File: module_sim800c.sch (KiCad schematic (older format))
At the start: 31 parts

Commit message: complete schematic
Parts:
- removed J?: LEMO2, symbol LEMO2
- removed P?: simcard, FCI_7111S2015X02LF, symbol 7111S2015X02LF
- J5: renamed from J?; value LEMO2 -> ANTEN
- gave numbers to parts that had none: 28
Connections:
- net labels added: +5V, RXD-01, TXD-01
- net labels removed: 5V, RXD, TXD
- no-connect marks 38 -> 36

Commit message: edit module sim800c
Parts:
- removed C10, C9: 22pF, symbol C
- removed C11, C12: 104, symbol C
- removed C7: C, symbol C
- removed D3: LED, symbol LED
- removed J6: CONN_01X04, symbol CONN_01X04
- removed P2: simcard, FCI_7111S2015X02LF, symbol 7111S2015X02LF
- removed R15: 1K, symbol R
- removed R16: R, symbol R
- removed R18, R19, R20, R21: 5,6K, symbol R
- removed R22, R23: 10K, symbol R
- removed R24: 330, symbol R
- added D3: D_TVS, Diodes_SMD:D_0603, symbol D_TVS
- added J?: SIM_Card, footprint:cardsim, symbol SIM_Card
- added SW1: SW_Push, symbol SW_Push
- added U8: SP1001, footprint:SP1001, symbol SP1001
- C5, C6, C8: footprint (none) -> footprint:C_0603
- D4: footprint (none) -> LEDs:LED_0603
- J7: footprint (none) -> Pin_Headers:Pin_Header_Angled_1x04_Pitch1.27mm
- R12, R13: value 1k -> 100; footprint (none) -> footprint:R_0603
- R14: value 1K -> 100; footprint (none) -> footprint:R_0603
- R17, R25: footprint (none) -> footprint:R_0603
- U3: footprint . -> footprint:sim800c
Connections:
- net labels added: +3V3, CTS, DCD, DTR, RI, RTS
- net labels removed: +5V
- wire segments 47 -> 56
- no-connect marks 36 -> 23
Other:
- moved on the sheet: C6, C8, D4, J7, R17, R25

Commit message: edit module sim800c
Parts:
- removed J?: SIM_Card, footprint:cardsim, symbol SIM_Card
- removed U3: SIM800C-RESCUE-esp32-gateway-hw, footprint:sim800c, symbol SIM800C-RESCUE-esp32-gateway-hw
- removed U8: SP1001, footprint:SP1001, symbol SP1001
- added J?: SIM_Card, symbol SIM_Card
- added U?: SIM800C-RESCUE-esp32-gateway-hw, ., symbol SIM800C-RESCUE-esp32-gateway-hw
- added U?: SP1001, symbol SP1001
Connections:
- wire segments 56 -> 55
- no-connect marks 23 -> 24
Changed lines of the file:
@@
 LIBS:zetex
 LIBS:Zilog
-LIBS:cardslot
 LIBS:esp32-wrover-v3
 LIBS:lm2596
@@
 LIBS:MOSFET-P
 LIBS:OPL-Inductor
-LIBS:sim800c
 LIBS:tc1264
 LIBS:neo-6m
 LIBS:Sim800c
 LIBS:sp1001
-LIBS:sim_card_holder
 LIBS:esp32-gateway-hw-cache
 EELAYER 25 0
@@
 	0    -1   -1   0
 $EndComp
-$Comp
-L SIM800C-RESCUE-esp32-gateway-hw U3
-U 1 1 59DD0550
-P 5850 3300
-F 0 "U3" H 5149 4521 50  0000 L BNN
-F 1 "SIM800C-RESCUE-esp32-gateway-hw" H 5149 1877 50  0000 L BNN
-F 2 "footprint:sim800c" H 7650 2800 50  0001 L BNN
-F 3 "." H 6900 3450 50  0001 L BNN
-F 4 "." H 5550 3800 50  0001 L BNN "Availability"
-F 5 "SIM800C" H 5700 3450 50  0001 L BNN "MP"
-F 6 "." H 5700 3100 50  0001 L BNN "Price"
-F 7 "." H 5750 3100 50  0001 L BNN "Package"
-F 8 "." H 5850 3300 50  0001 L BNN "MF"
-	1    5850 3300
-	1    0    0    -1
-$EndComp
 NoConn ~ 6750 3400
 $Comp
@@
 RI
 $Comp
-L SP1001 U8
-U 1 1 59DD10E8
-P 7500 3550
-F 0 "U8" H 7450 3250 60  0000 C CNN
-F 1 "SP1001" H 7450 4000 60  0000 C CNN
-F 2 "footprint:SP1001" H 7500 3550 60  0001 C CNN
-F 3 "" H 7500 3550 60  0001 C CNN
-	1    7500 3550
-	1    0    0    -1
-$EndComp
-$Comp
 L GND #PWR026
 U 1 1 59DD114F
@@
 	4700 2300 4950 2300
 $Comp
+L SIM800C-RESCUE-esp32-gateway-hw U?
+U 1 1 59DD1931
+P 5850 3300
+F 0 "U?" H 5149 4521 50  0000 L BNN
+F 1 "SIM800C-RESCUE-esp32-gateway-hw" H 5149 1877 50  0000 L BNN
+F 2 "." H 7650 2800 50  0001 L BNN
+F 3 "." H 6900 3450 50  0001 L BNN
+F 4 "." H 5550 3800 50  0001 L BNN "Availability"
+F 5 "SIM800C" H 5700 3450 50  0001 L BNN "MP"
+F 6 "." H 5700 3100 50  0001 L BNN "Price"
+F 7 "." H 5750 3100 50  0001 L BNN "Package"
+F 8 "." H 5850 3300 50  0001 L BNN "MF"
+	1    5850 3300
+	1    0    0    -1
+$EndComp
+$Comp
 L SIM_Card J?
-U 1 1 59DD0C98
+U 1 1 59DD1A9A
 P 8350 2900
-AR Path="/59DD0C98" Ref="J?"  Part="1"
-AR Path="/59DC8035/59DD0C98" Ref="J?"  Part="1"
 F 0 "J?" H 8250 3400 50  0000 R CNN
 F 1 "SIM_Card" H 8300 3300 50  0000 R CNN
-F 2 "footprint:cardsim" H 8350 3250 50  0000 C CNN
+F 2 "" H 8350 3250 50  0000 C CNN
 F 3 "" H 8300 2900 50  0000 C CNN
 	1    8350 2900
 	1    0    0    -1
 $EndComp
-Wire Wire Line
-	7850 3100 7850 3000
+NoConn ~ 7850 3000
+$Comp
+L SP1001 U?
+U 1 1 59DD1ECF
+P 7500 3550
+F 0 "U?" H 7450 3250 60  0000 C CNN
+F 1 "SP1001" H 7450 4000 60  0000 C CNN
+F 2 "" H 7500 3550 60  0001 C CNN
+F 3 "" H 7500 3550 60  0001 C CNN
+	1    7500 3550
+	1    0    0    -1
+$EndComp
 $EndSCHEMATC

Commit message: fix mach nap
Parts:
- J5: symbol LEMO2 -> LEMO2-RESCUE-esp32-gateway-hw
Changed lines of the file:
@@
 LIBS:contrib
 LIBS:valves
+LIBS:esp32-wrover-v3
 LIBS:Symbols_DCDC-ACDC-Converter_RevC_20Jul2012
 LIBS:Symbols_EN60617_13Mar2013
@@
 LIBS:ftdi
 LIBS:gennum
+LIBS:graphic_symbols
 LIBS:hc11
+LIBS:infineon
+LIBS:intersil
 LIBS:ir
 LIBS:Lattice
 LIBS:leds
+LIBS:LEM
+LIBS:logic_programmable
 LIBS:maxim
 LIBS:mechanical
@@
 LIBS:relays
 LIBS:rfcom
+LIBS:RFSolutions
 LIBS:sensors
 LIBS:silabs
@@
 LIBS:zetex
 LIBS:Zilog
-LIBS:esp32-wrover-v3
+LIBS:CP2102
+LIBS:ESP8266
+LIBS:esp-uno
+LIBS:esp-wroom-32
+LIBS:microsd_socket
+LIBS:microsd_spi_cd
+LIBS:MOSFET-N
+LIBS:MOSFET-P
+LIBS:open-project
+LIBS:tc1264
+LIBS:tom_kicad
+LIBS:usb-b
+LIBS:usb_mini_b
+LIBS:w_device
 LIBS:lm2596
 LIBS:mcp73831
-LIBS:MOSFET-P
 LIBS:OPL-Inductor
-LIBS:tc1264
 LIBS:neo-6m
 LIBS:Sim800c
@@
 $EndComp
 $Comp
-L LEMO2 J5
+L LEMO2-RESCUE-esp32-gateway-hw J5
 U 1 1 59DC618A
 P 3700 4000
+AR Path="/59DC618A" Ref="J5"  Part="1"
+AR Path="/59DC8035/59DC618A" Ref="J5"  Part="1"
 F 0 "J5" H 3700 4200 50  0000 C CNN
 F 1 "ANTEN" H 3700 3800 50  0000 C CNN

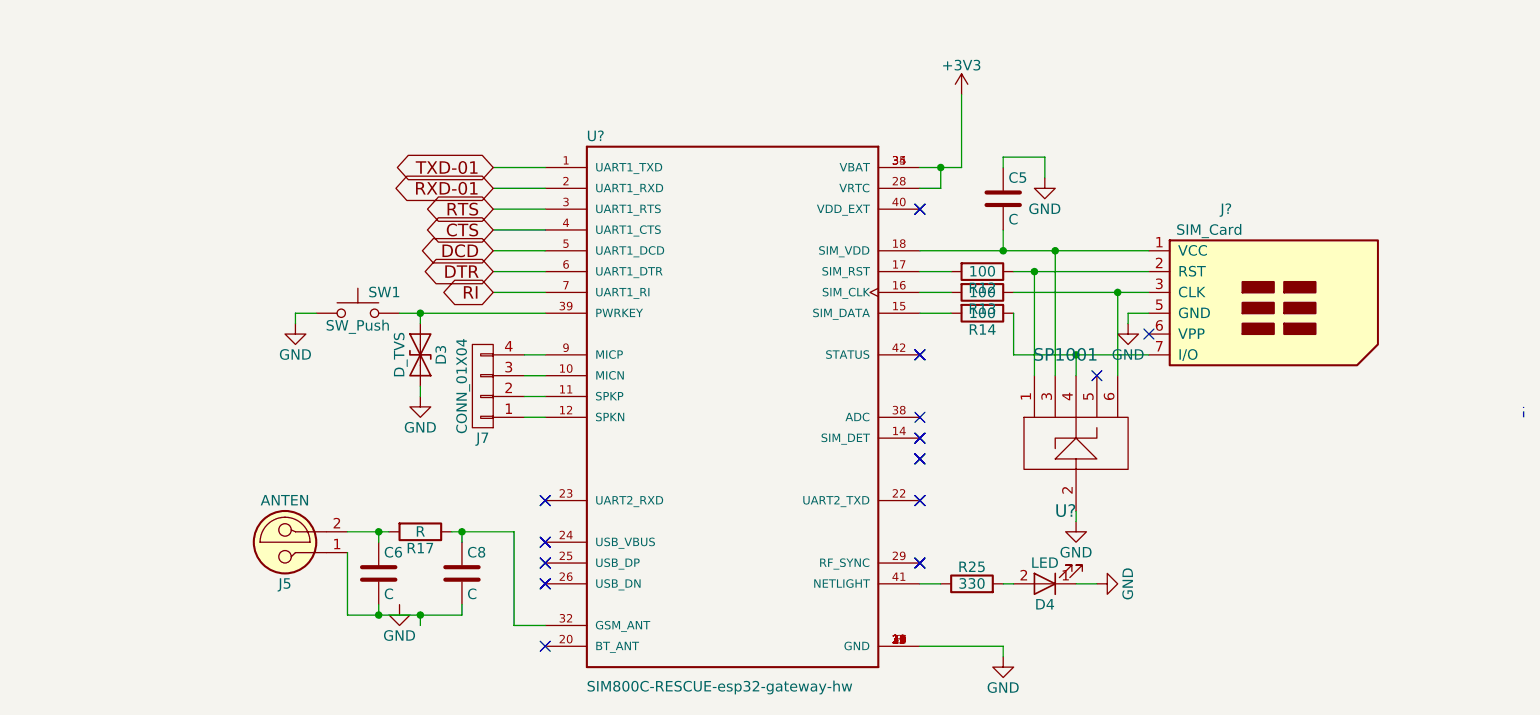
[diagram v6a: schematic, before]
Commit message: update layout
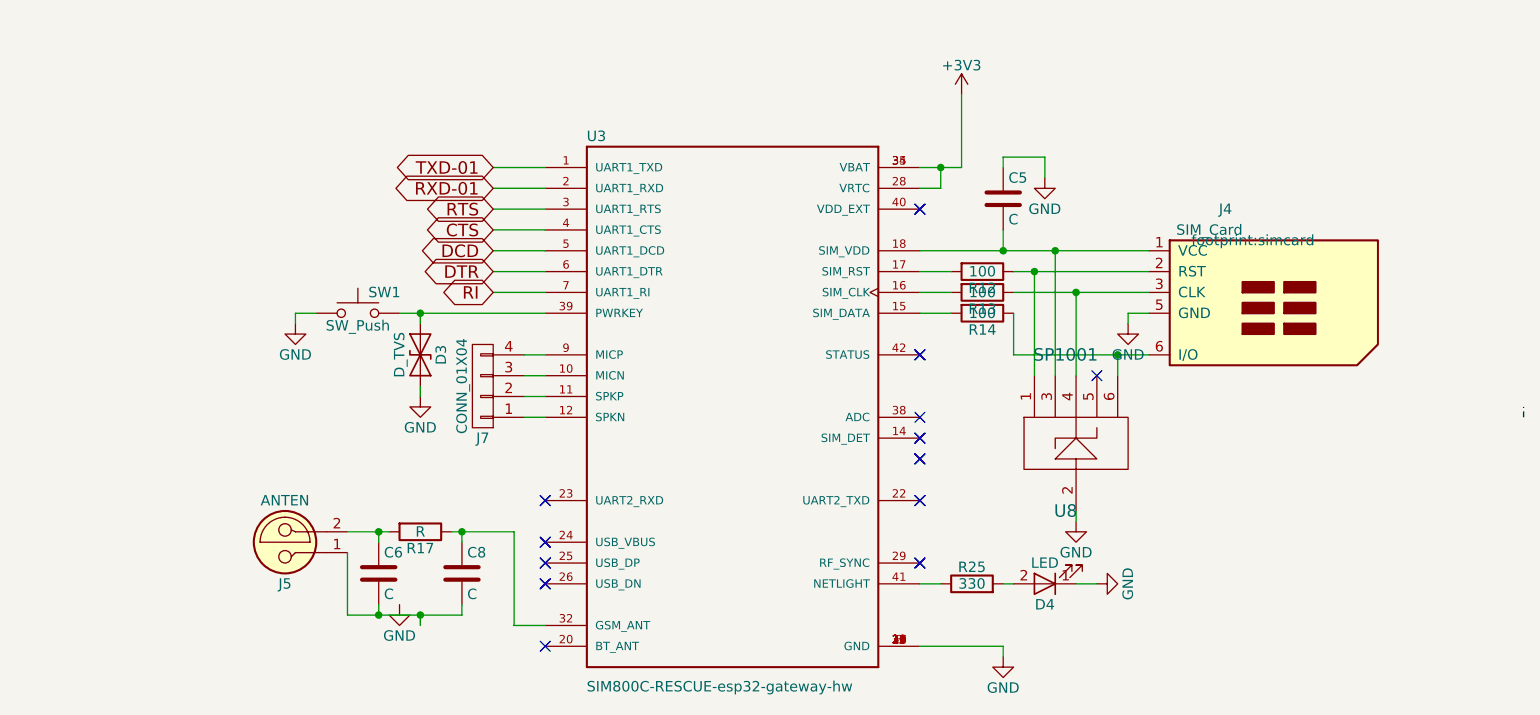
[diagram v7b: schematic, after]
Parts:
- removed J?: SIM_Card, symbol SIM_Card
- added J4: SIM_Card, footprint:simcard, symbol SIM_Card-RESCUE-esp32-gateway-hw
- D3: footprint Diodes_SMD:D_0603 -> Diodes_SMD:D_1206
- J5: footprint (none) -> Pin_Headers:Pin_Header_Straight_1x02_Pitch1.00mm
- SW1: footprint (none) -> footprint:Tact_Switch_TS6X3.6
- U3: renamed from U?; footprint . -> footprint:sim800c
- U8: renamed from U?; footprint (none) -> footprint:SP1001
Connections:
- net GND: now also J4.5 (GND)
- net at R12.1, U8.1: now also J4.2 (RST)
- net at R13.1: now also U8.4, J4.3 (CLK); no longer U8.6
- net at R14.1: now also U8.6, J4.6 (I/O); no longer U8.4
- net at C5.2, U3.18 (SIM_VDD), U8.3: now also J4.1 (VCC)
- no-connect marks 24 -> 23
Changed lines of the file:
@@
 LIBS:contrib
 LIBS:valves
-LIBS:esp32-wrover-v3
 LIBS:Symbols_DCDC-ACDC-Converter_RevC_20Jul2012
 LIBS:Symbols_EN60617_13Mar2013
@@
 LIBS:ftdi
 LIBS:gennum
-LIBS:graphic_symbols
 LIBS:hc11
-LIBS:infineon
-LIBS:intersil
 LIBS:ir
 LIBS:Lattice
 LIBS:leds
-LIBS:LEM
-LIBS:logic_programmable
 LIBS:maxim
 LIBS:mechanical
@@
 LIBS:relays
 LIBS:rfcom
-LIBS:RFSolutions
 LIBS:sensors
 LIBS:silabs
@@
 LIBS:zetex
 LIBS:Zilog
-LIBS:CP2102
-LIBS:ESP8266
-LIBS:esp-uno
-LIBS:esp-wroom-32
-LIBS:microsd_socket
-LIBS:microsd_spi_cd
-LIBS:MOSFET-N
-LIBS:MOSFET-P
-LIBS:open-project
-LIBS:tc1264
-LIBS:tom_kicad
-LIBS:usb-b
-LIBS:usb_mini_b
-LIBS:w_device
+LIBS:esp32-wrover-v3
 LIBS:lm2596
 LIBS:mcp73831
+LIBS:MOSFET-P
 LIBS:OPL-Inductor
+LIBS:tc1264
 LIBS:neo-6m
 LIBS:Sim800c
+LIBS:sim_card_holder
 LIBS:sp1001
 LIBS:esp32-gateway-hw-cache
@@
 $Descr A4 11693 8268
 encoding utf-8
-Sheet 3 4
+Sheet 2 4
 Title ""
 Date ""
@@
 NoConn ~ 6750 3800
 $Comp
-L GND #PWR020
+L GND #PWR010
 U 1 1 59DC6183
 P 7150 4550
-F 0 "#PWR020" H 7150 4300 50  0001 C CNN
+F 0 "#PWR010" H 7150 4300 50  0001 C CNN
 F 1 "GND" H 7150 4400 50  0000 C CNN
 F 2 "" H 7150 4550 50  0001 C CNN
@@
 $EndComp
 $Comp
-L GND #PWR021
+L GND #PWR011
 U 1 1 59DC6189
 P 4250 4300
-F 0 "#PWR021" H 4250 4050 50  0001 C CNN
+F 0 "#PWR011" H 4250 4050 50  0001 C CNN
 F 1 "GND" H 4250 4150 50  0000 C CNN
 F 2 "" H 4250 4300 50  0001 C CNN
@@
 AR Path="/59DC618A" Ref="J5"  Part="1"
 AR Path="/59DC8035/59DC618A" Ref="J5"  Part="1"
+AR Path="/59DDD837/59DC618A" Ref="J5"  Part="1"
+AR Path="/59DDC248/59DC618A" Ref="J5"  Part="1"
 F 0 "J5" H 3700 4200 50  0000 C CNN
 F 1 "ANTEN" H 3700 3800 50  0000 C CNN
-F 2 "" H 3700 4000 50  0001 C CNN
+F 2 "Pin_Headers:Pin_Header_Straight_1x02_Pitch1.00mm" H 3700 4000 50  0001 C CNN
 F 3 "" H 3700 4000 50  0001 C CNN
 	1    3700 4000
@@
 $EndComp
 $Comp
-L +3V3 #PWR022
+L +3V3 #PWR012
 U 1 1 59DCE5F6
 P 6950 1850
-F 0 "#PWR022" H 6950 1700 50  0001 C CNN
+F 0 "#PWR012" H 6950 1700 50  0001 C CNN
 F 1 "+3V3" H 6950 1990 50  0000 C CNN
 F 2 "" H 6950 1850 50  0001 C CNN
@@
 $EndComp
 $Comp
-L GND #PWR023
+L GND #PWR013
 U 1 1 59DCFA55
 P 7600 4200
-F 0 "#PWR023" H 7600 3950 50  0001 C CNN
+F 0 "#PWR013" H 7600 3950 50  0001 C CNN
 F 1 "GND" H 7600 4050 50  0000 C CNN
 F 2 "" H 7600 4200 50  0001 C CNN
@@
 F 0 "D3" H 4350 3200 50  0000 C CNN
 F 1 "D_TVS" H 4350 3000 50  0000 C CNN
-F 2 "Diodes_SMD:D_0603" H 4350 3100 50  0001 C CNN
+F 2 "Diodes_SMD:D_1206" H 4350 3100 50  0001 C CNN
 F 3 "" H 4350 3100 50  0001 C CNN
 	1    4350 3100
@@
 F 0 "SW1" H 4100 3000 50  0000 L CNN
 F 1 "SW_Push" H 4050 2840 50  0000 C CNN
-F 2 "" H 4050 3100 50  0001 C CNN
+F 2 "footprint:Tact_Switch_TS6X3.6" H 4050 3100 50  0001 C CNN
 F 3 "" H 4050 3100 50  0001 C CNN
 	1    4050 2900
@@
 $EndComp
 $Comp
-L GND #PWR024
+L GND #PWR014
 U 1 1 59DD0AE0
 P 3750 2950
-F 0 "#PWR024" H 3750 2700 50  0001 C CNN
+F 0 "#PWR014" H 3750 2700 50  0001 C CNN
 F 1 "GND" H 3750 2800 50  0000 C CNN
 F 2 "" H 3750 2950 50  0001 C CNN
@@
 $EndComp
 $Comp
-L GND #PWR025
+L GND #PWR015
 U 1 1 59DD0B6C
 P 4350 3300
-F 0 "#PWR025" H 4350 3050 50  0001 C CNN
+F 0 "#PWR015" H 4350 3050 50  0001 C CNN
 F 1 "GND" H 4350 3150 50  0000 C CNN
 F 2 "" H 4350 3300 50  0001 C CNN
@@
 RI
 $Comp
-L GND #PWR026
+L GND #PWR016
 U 1 1 59DD114F
 P 7500 3900
-F 0 "#PWR026" H 7500 3650 50  0001 C CNN
+F 0 "#PWR016" H 7500 3650 50  0001 C CNN
 F 1 "GND" H 7500 3750 50  0000 C CNN
 F 2 "" H 7500 3900 50  0001 C CNN
@@
 $EndComp
 $Comp
-L GND #PWR027
+L GND #PWR017
 U 1 1 59DD1317
 P 7750 2950
-F 0 "#PWR027" H 7750 2700 50  0001 C CNN
+F 0 "#PWR017" H 7750 2700 50  0001 C CNN
 F 1 "GND" H 7750 2800 50  0000 C CNN
 F 2 "" H 7750 2950 50  0001 C CNN
@@
 	7200 2900 7200 3100
 Wire Wire Line
-	7200 3100 7850 3100
-Wire Wire Line
 	7300 3200 7300 2700
 Connection ~ 7300 2700
-Wire Wire Line
-	7500 3100 7500 3200
-Connection ~ 7500 3100
-Wire Wire Line
-	7700 3200 7700 2800
-Connection ~ 7700 2800
 Wire Wire Line
 	6750 2600 7850 2600
@@
 Connection ~ 7150 2600
 $Comp
-L GND #PWR028
+L GND #PWR018
 U 1 1 59DD1C11
 P 7350 2250
-F 0 "#PWR028" H 7350 2000 50  0001 C CNN
+F 0 "#PWR018" H 7350 2000 50  0001 C CNN
 F 1 "GND" H 7350 2100 50  0000 C CNN
 F 2 "" H 7350 2250 50  0001 C CNN
@@
 	4700 2300 4950 2300
 $Comp
-L SIM800C-RESCUE-esp32-gateway-hw U?
+L SIM800C-RESCUE-esp32-gateway-hw U3
 U 1 1 59DD1931
 P 5850 3300
-F 0 "U?" H 5149 4521 50  0000 L BNN
+F 0 "U3" H 5149 4521 50  0000 L BNN
 F 1 "SIM800C-RESCUE-esp32-gateway-hw" H 5149 1877 50  0000 L BNN
-F 2 "." H 7650 2800 50  0001 L BNN
+F 2 "footprint:sim800c" H 7650 2800 50  0001 L BNN
 F 3 "." H 6900 3450 50  0001 L BNN
 F 4 "." H 5550 3800 50  0001 L BNN "Availability"
@@
 $EndComp
 $Comp
-L SIM_Card J?
-U 1 1 59DD1A9A
+L SP1001 U8
+U 1 1 59DD1ECF
+P 7500 3550
+F 0 "U8" H 7450 3250 60  0000 C CNN
+F 1 "SP1001" H 7450 4000 60  0000 C CNN
+F 2 "footprint:SP1001" H 7500 3550 60  0001 C CNN
+F 3 "" H 7500 3550 60  0001 C CNN
+	1    7500 3550
+	1    0    0    -1
+$EndComp
+$Comp
+L SIM_Card-RESCUE-esp32-gateway-hw J4
+U 1 1 59DDD9DD
 P 8350 2900
-F 0 "J?" H 8250 3400 50  0000 R CNN
+F 0 "J4" H 8250 3400 50  0000 R CNN
 F 1 "SIM_Card" H 8300 3300 50  0000 R CNN
-F 2 "" H 8350 3250 50  0000 C CNN
+F 2 "footprint:simcard" H 8350 3250 50  0000 C CNN
 F 3 "" H 8300 2900 50  0000 C CNN
 	1    8350 2900
 	1    0    0    -1
 $EndComp
-NoConn ~ 7850 3000
-$Comp
-L SP1001 U?
-U 1 1 59DD1ECF
-P 7500 3550
-F 0 "U?" H 7450 3250 60  0000 C CNN
-F 1 "SP1001" H 7450 4000 60  0000 C CNN
-F 2 "" H 7500 3550 60  0001 C CNN
-F 3 "" H 7500 3550 60  0001 C CNN
-	1    7500 3550
-	1    0    0    -1
-$EndComp
+Wire Wire Line
+	7200 3100 7850 3100
+Wire Wire Line
+	7500 3200 7500 2800
+Connection ~ 7500 2800
+Wire Wire Line
+	7700 3200 7700 3100
+Connection ~ 7700 3100
 $EndSCHEMATC
